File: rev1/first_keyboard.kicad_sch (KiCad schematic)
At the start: 80 parts, among them SW1 SW_Push, SW10 SW_Push, SW11 SW_Push, SW12 SW_Push, SW13 SW_Push, SW14 SW_Push, SW15 SW_Push, SW16 SW_Push, SW17 SW_Push, SW18 SW_Push, SW19 SW_Push, SW2 SW_Push, SW20 SW_Push, SW21 SW_Push, SW22 SW_Push, SW23 SW_Push, SW24 SW_Push, SW25 SW_Push, SW26 SW_Push, SW27 SW_Push, SW28 SW_Push, SW29 SW_Push, SW3 SW_Push, SW30 SW_Push, SW31 SW_Push, SW32 SW_Push, SW33 SW_Push, SW34 SW_Push, SW35 SW_Push, SW36 SW_Push, SW37 SW_Push, SW38 SW_Push, SW39 SW_Push, SW4 SW_Push, SW40 SW_Push, SW5 SW_Push, SW6 SW_Push, SW7 SW_Push, SW8 SW_Push, SW9 SW_Push, U1 Pico

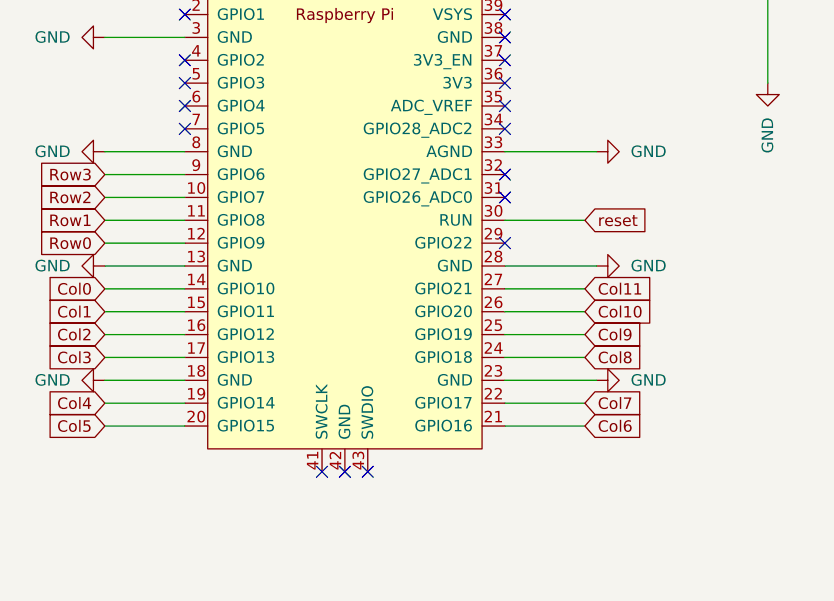
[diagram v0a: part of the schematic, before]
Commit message: fix: ボードの反転を意識してタグを振りなおした
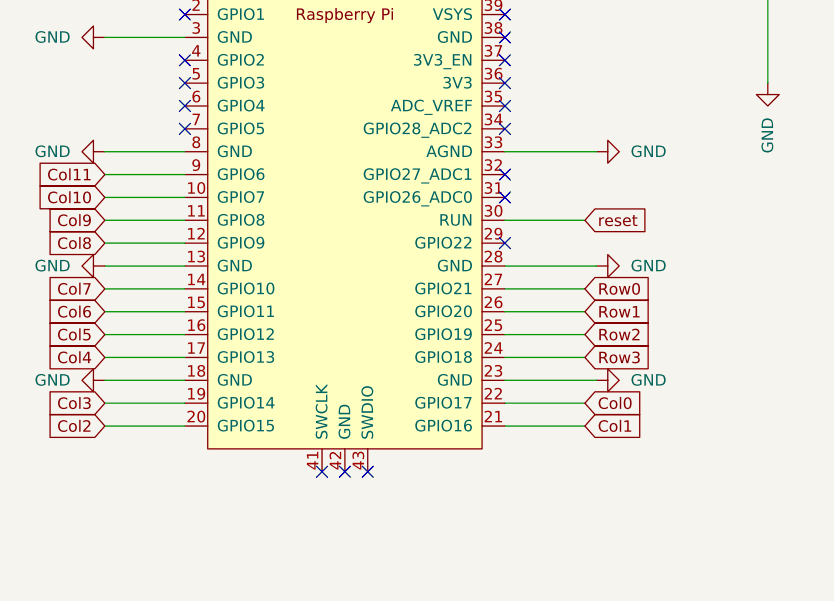
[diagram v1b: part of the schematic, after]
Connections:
- net Col0: now also U1.22 (GPIO17); no longer U1.14 (GPIO10)
- net Col1: now also U1.21 (GPIO16); no longer U1.15 (GPIO11)
- net Col10: now also U1.10 (GPIO7); no longer U1.26 (GPIO20)
- net Col11: now also U1.9 (GPIO6); no longer U1.27 (GPIO21)
- net Col2: now also U1.20 (GPIO15); no longer U1.16 (GPIO12)
- net Col3: now also U1.19 (GPIO14); no longer U1.17 (GPIO13)
- net Col4: now also U1.17 (GPIO13); no longer U1.19 (GPIO14)
- net Col5: now also U1.16 (GPIO12); no longer U1.20 (GPIO15)
- net Col6: now also U1.15 (GPIO11); no longer U1.21 (GPIO16)
- net Col7: now also U1.14 (GPIO10); no longer U1.22 (GPIO17)
- net Col8: now also U1.12 (GPIO9); no longer U1.24 (GPIO18)
- net Col9: now also U1.11 (GPIO8); no longer U1.25 (GPIO19)
- net Row0: now also U1.27 (GPIO21); no longer U1.12 (GPIO9)
- net Row1: now also U1.26 (GPIO20); no longer U1.11 (GPIO8)
- net Row2: now also U1.25 (GPIO19); no longer U1.10 (GPIO7)
- net Row3: now also U1.24 (GPIO18); no longer U1.9 (GPIO6)
